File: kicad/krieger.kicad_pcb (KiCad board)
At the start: 2 copper layers, 80 x 47 mm, 26 parts, among them J1 USB-C, SW1 Reset, U1 LP5907MFX-3.3, U2 SRV05-4, U3 STM32F072C8Tx, U4 proto-area

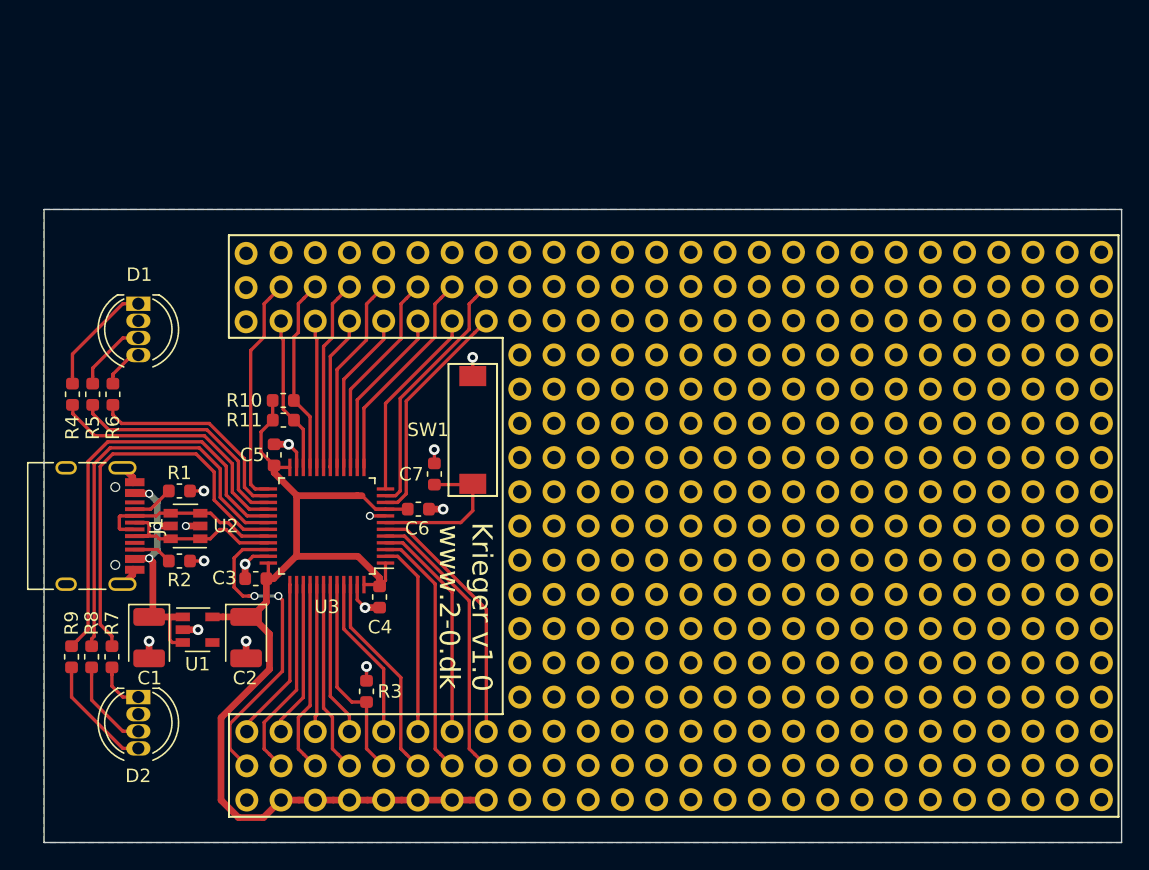
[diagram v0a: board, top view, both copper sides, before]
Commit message: Krieger_v2.00
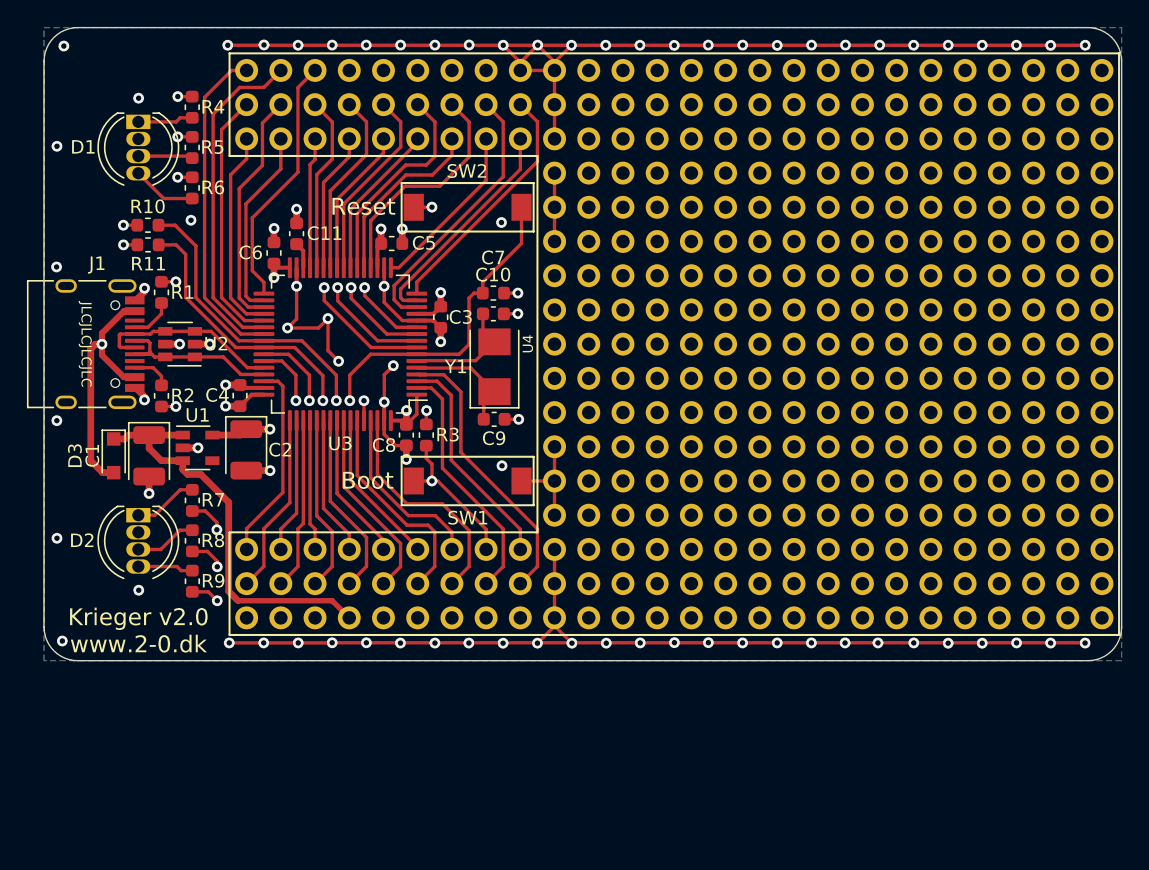
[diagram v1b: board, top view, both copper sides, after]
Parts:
- added C10: 16p, Capacitor_SMD:C_0603_1608Metric, F.Cu at (153.4, 97.8)
- added C11: 1u, Capacitor_SMD:C_0603_1608Metric, F.Cu at (138.8, 91.8)
- added C8: 100n, Capacitor_SMD:C_0603_1608Metric, F.Cu at (146.9, 106.8)
- added C9: 16p, Capacitor_SMD:C_0603_1608Metric, F.Cu at (153.4, 105.6)
- added D3: 1N5819WS, Diode_SMD:D_SOD-323_HandSoldering, F.Cu at (125.2, 108.3)
- added SW2: Reset, krieger:TACT-SWITCH, F.Cu at (151.4, 89.8)
- added Y1: 8 MHz, Crystal:Crystal_SMD_5032-2Pin_5.0x3.2mm, F.Cu at (153.4, 101.7)
- R4, R5, R6, R7, R8, R9: value 470 -> 1k
- SW1: value Reset -> Boot
- U3: value STM32F072C8Tx -> STM32F446RETx; footprint Package_QFP:LQFP-48_7x7mm_P0.5mm -> Package_QFP:LQFP-64_10x10mm_P0.5mm
- moved C3 23.8 mm to (149.4, 98.0), turned to 270 degrees
- moved R4 23.1 mm to (131.0, 82.4), turned to 270 degrees
- moved C6 21.8 mm to (137.1, 93.2), turned to 90 degrees
- moved R5 19.8 mm to (131.0, 85.4), turned to 270 degrees
- moved R3 19.5 mm to (148.4, 106.8)
- moved C4 18.2 mm to (134.6, 103.8), turned to 90 degrees
- moved C5 18.0 mm to (145.8, 92.5), turned to 0 degrees
- moved R11 16.4 mm to (127.7, 92.6)
- moved R10 16.4 mm to (127.7, 91.2)
- moved R6 16.4 mm to (131.0, 88.4), turned to 270 degrees
- moved R1 14.8 mm to (128.7, 96.2), turned to 270 degrees
- moved C7 14.1 mm to (153.4, 96.2), turned to 0 degrees
- moved C2 13.9 mm to (135.0, 107.8)
- moved U3 13.5 mm to (142.0, 100.0)
- moved U2 13.5 mm to (130.1, 100.0)
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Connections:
- C1 pad 1: vusb -> +5V
- J1 pad S1: GND -> Net-(J1-PadS1)
- R10 pad 1: i2c_scl -> sda3
- R11 pad 1: i2c_sda -> scl3
- R4 pad 1: led1_red -> hmi1_red
- R5 pad 1: led1_green -> hmi1_green
- R6 pad 1: led1_blue -> hmi1_blue
- R7 pad 1: led2_red -> hmi2_red
- R8 pad 1: led2_green -> hmi2_green
- R9 pad 1: led2_blue -> hmi2_blue
- SW1 pad 1: nrst -> boot0
- SW1 pad 2: GND -> +3V3
- U1 pad 1: vusb -> +5V
- U1 pad 3: vusb -> +5V
- U3 pad 10: pa0 -> pc2
- U3 pad 11: pa1 -> pc3
- U3 pad 12: uart_tx -> GND
- U3 pad 13: uart_rx -> +3V3
- U3 pad 14: pa4 -> pa0
- U3 pad 15: spi_sck -> pa1
- U3 pad 16: spi_miso -> pa2
- U3 pad 17: spi_mosi -> pa3
- U3 pad 18: pb0 -> GND
- U3 pad 19: pb1 -> +3V3
- U3 pad 20: pb2 -> pa4
- U3 pad 21: i2c_scl -> pa5
- U3 pad 22: i2c_sda -> pa6
- U3 pad 23: GND -> pa7
- U3 pad 24: +3V3 -> pc4
- U3 pad 25: pb12 -> pc5
- U3 pad 26: led1_blue -> pb0
- U3 pad 27: led1_green -> pb1
- U3 pad 28: led1_red -> pb2
- U3 pad 29: led2_blue -> pb10
- U3 pad 30: led2_green -> vcap_1
- U3 pad 31: led2_red -> GND
- U3 pad 32: usb_dm -> +3V3
- U3 pad 33: usb_dp -> pb12
- U3 pad 34: swdio -> pb13
- U3 pad 35: GND -> pb14
- U3 pad 36: +3V3 -> pb15
- U3 pad 37: swclk -> hmi1_blue
- U3 pad 38: pa15 -> hmi1_green
- U3 pad 39: pb3 -> hmi1_red
- U3 pad 40: pb4 -> sda3
- U3 pad 41: pb5 -> scl3
- U3 pad 42: pb6 -> tx1
- U3 pad 43: pb7 -> rx1
- U3 pad 44: boot0 -> usb_dm
- U3 pad 45: pb8 -> usb_dp
- U3 pad 46: pb9 -> swdio
- U3 pad 5: pf0 -> Net-(C9-Pad1)
- U3 pad 6: pf1 -> Net-(C10-Pad1)
- U3 pad 8: GND -> pc0
- U3 pad 9: +3V3 -> pc1
- U4 pad 10: spi_mosi -> swclk
- U4 pad 11: pa4 -> hmi2_green
- U4 pad 12: spi_sck -> hmi2_blue
- U4 pad 13: uart_tx -> pb3
- U4 pad 14: uart_rx -> pb5
- U4 pad 15: pa0 -> pb7
- U4 pad 16: pa1 -> pb9
- U4 pad 17: pf0 -> pc13
- U4 pad 18: pf1 -> pc15
- U4 pad 19: pc14 -> swdio
- U4 pad 20: pc15 -> pa15
- U4 pad 21: pb9 -> hmi2_red
- U4 pad 22: pc13 -> pd2
- U4 pad 23: boot0 -> pb4
- U4 pad 24: pb8 -> pb6
- U4 pad 25: pb6 -> pb8
- U4 pad 26: pb7 -> boot0
- U4 pad 27: pb4 -> pc14
- U4 pad 28: pb5 -> pb15
- U4 pad 29: pa15 -> pb13
- U4 pad 3: i2c_sda -> GND
- U4 pad 30: pb3 -> pb10
- U4 pad 31: swdio -> pb1
- U4 pad 32: swclk -> pc5
- U4 pad 4: pb12 -> +5V
- U4 pad 5: pb2 -> rx1
- U4 pad 6: i2c_scl -> tx1
- U4 pad 7: pb0 -> scl3
- U4 pad 8: pb1 -> sda3
- U4 pad 9: spi_miso -> nrst
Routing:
- net GND: track 24.5 -> 204.7 mm, vias 14 -> 89
- net sda3: track 0.00 -> 43.9 mm, vias 0 -> 1
- net scl3: track 0.00 -> 40.0 mm, vias 0 -> 1
- net hmi1_green: track 0.00 -> 36.0 mm, vias 0 -> 1
- net nrst: track 11.7 -> 47.1 mm, vias 0 -> 1
- net led2_blue: track 31.7 -> 0.00 mm
- net hmi1_red: track 0.00 -> 31.3 mm, vias 0 -> 1
- net +5V: track 0.00 -> 30.6 mm
- net led2_green: track 30.6 -> 0.00 mm
- net led2_red: track 30.1 -> 0.00 mm
- net hmi1_blue: track 0.00 -> 28.6 mm, vias 0 -> 1
- net pc0: track 0.00 -> 26.2 mm, vias 0 -> 1
- net pc1: track 0.00 -> 25.6 mm, vias 0 -> 1
- net tx1: track 0.00 -> 25.4 mm, vias 0 -> 1
- net pc2: track 0.00 -> 24.9 mm, vias 0 -> 1
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- added copper zone on In2.Cu, net +3V3
- added copper zone on In1.Cu, net GND
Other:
- outline, holes or cut-outs redrawn
- copper layers 2 -> 4
- board text added: "Boot"
- board text added: "JLCJLCJLCJLC"
- board text added: "Krieger v2.0 www.2-0.dk"
- board text added: "Reset"
- board text removed: "Krieger v1.0 www.2-0.dk"

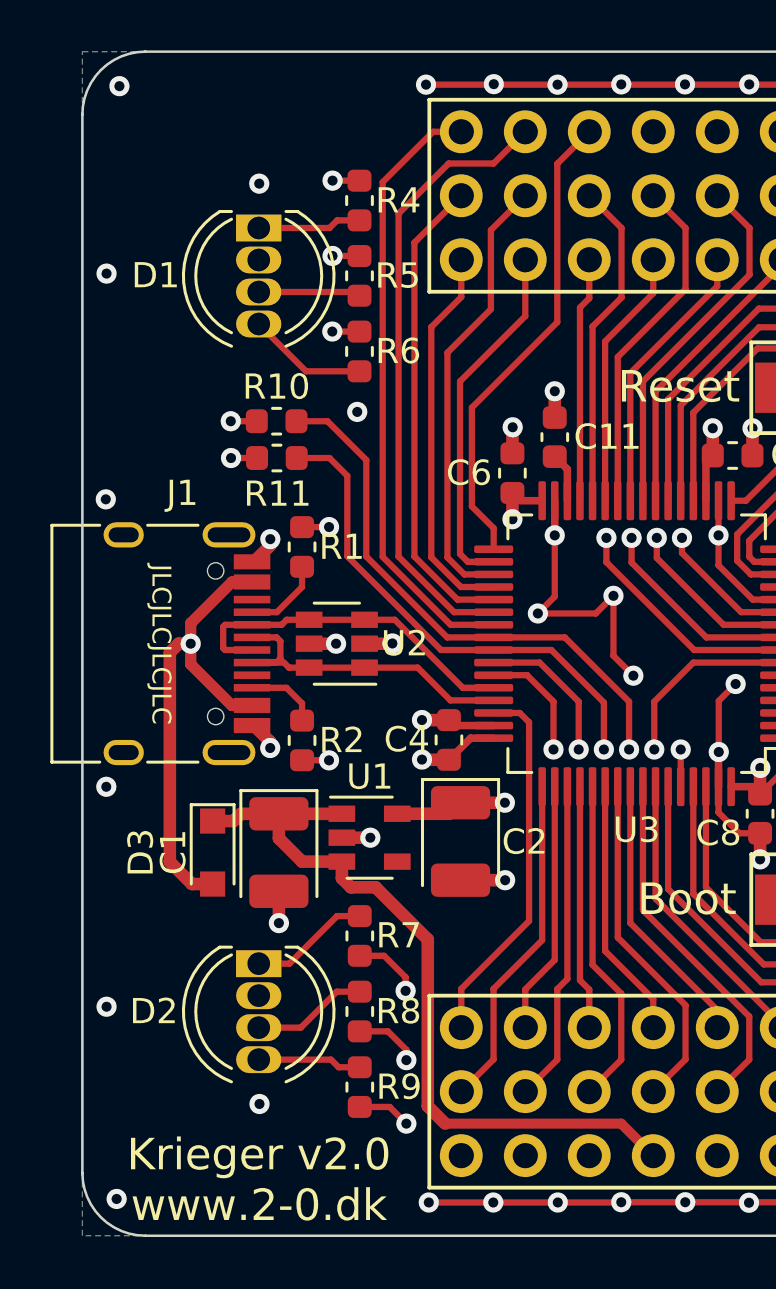
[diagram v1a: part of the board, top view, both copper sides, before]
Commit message: Krieger v2.00
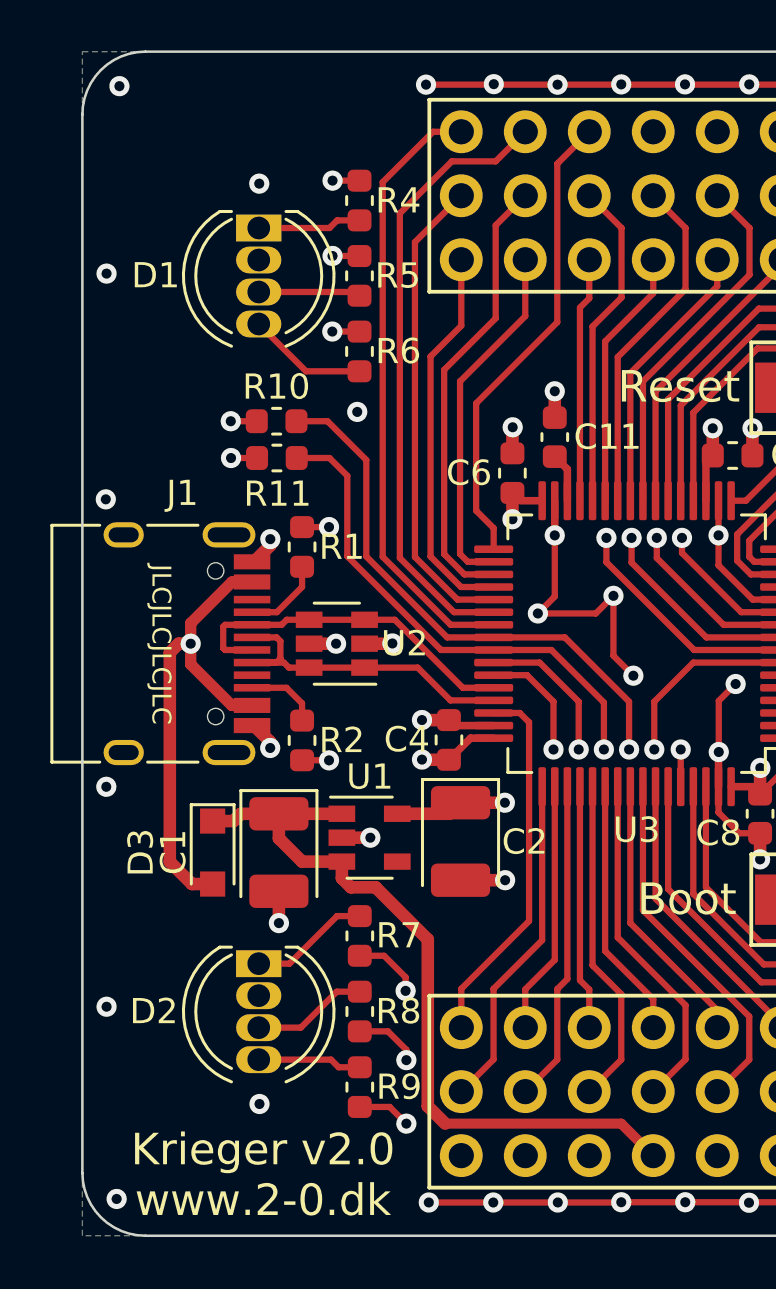
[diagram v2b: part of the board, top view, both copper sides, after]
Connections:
- U3 pad 35: pb14 -> hmi1_green
- U3 pad 36: pb15 -> hmi1_blue
- U3 pad 37: hmi1_blue -> pc6
- U3 pad 38: hmi1_green -> pc7
- U3 pad 53: hmi2_blue -> pc12
- U3 pad 57: pb5 -> hmi2_blue
- U4 pad 12: hmi2_blue -> pc12
- U4 pad 14: pb5 -> hmi2_blue
- U4 pad 28: pb15 -> hmi1_blue
- U4 pad 37: hmi1_blue -> pc6
- U4 pad 38: pb14 -> hmi1_green
- U4 pad 47: hmi1_green -> pc7
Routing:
- net pc7: track 0.00 -> 24.6 mm
- net pc6: track 0.00 -> 18.9 mm
- net pb14: track 17.8 -> 0.00 mm
- net pb15: track 15.3 -> 0.00 mm
- net pb5: track 14.4 -> 0.00 mm
- net pc12: track 0.00 -> 13.1 mm
- net hmi1_green: track 36.0 -> 27.6 mm
- net hmi2_blue: track 23.0 -> 29.4 mm
- net hmi1_blue: track 28.6 -> 22.7 mm
